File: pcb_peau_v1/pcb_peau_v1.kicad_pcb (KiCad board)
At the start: 2 copper layers, 76 x 75.7 mm, 27 parts, among them J1 Conn_01x05, J2 Conn_01x05, J3 Conn_01x02, J4 Conn_02x08_Top_Bottom, J5 Conn_02x12_Top_Bottom, U2 TLC274, U3 CD74HC4067SM, U4 CD74HC4067SM, U5 CD74HC4067SM, U6 CD74HC4067SM, U7 TLC274, U8 TLC274, U9 TLC274

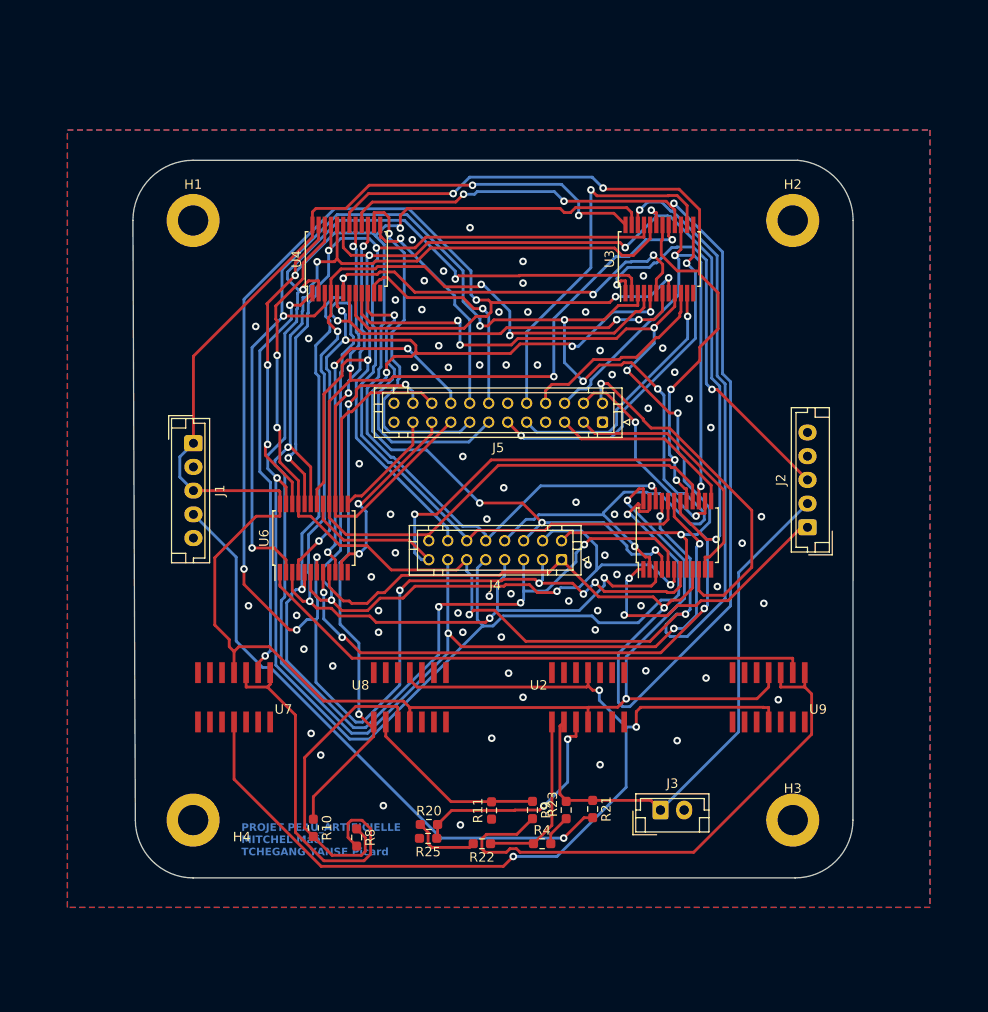
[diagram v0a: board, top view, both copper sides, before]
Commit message: pdb bulletproof
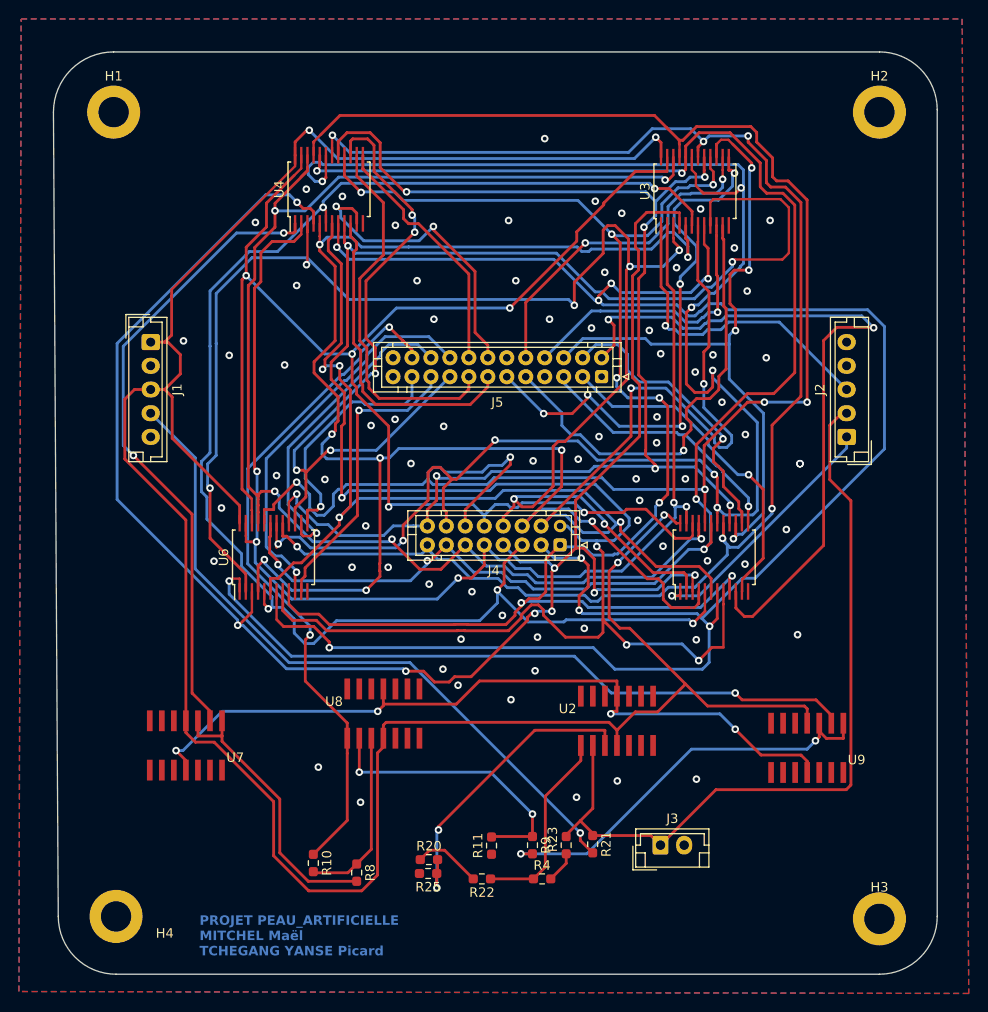
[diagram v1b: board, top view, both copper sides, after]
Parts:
- moved H2 14.6 mm to (247.7, 39.1)
- moved H1 14.2 mm to (166.9, 39.1)
- moved H3 13.9 mm to (247.7, 124.2)
- moved H4 13.0 mm to (167.1, 124.0)
- moved J1 11.6 mm to (170.8, 63.4)
- moved J2 10.4 mm to (244.2, 73.4)
- moved U3 8.07 mm to (228.2, 47.5)
- moved U4 7.58 mm to (189.6, 47.3)
- moved U7 7.18 mm to (174.5, 105.9)
- moved U9 6.71 mm to (240.0, 106.2)
- moved J5 4.79 mm to (218.3, 67.0)
- moved U6 4.71 mm to (183.7, 86.1)
- moved U5 4.54 mm to (230.2, 86.1)
- moved U2 3.93 mm to (220.0, 103.3)
- moved J3 3.71 mm to (224.6, 116.4)
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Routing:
- net Net-(J4-Pin_2): track 144.7 -> 210.5 mm, vias 9 -> 6
- net +5V: track 200.4 -> 262.6 mm
- net Net-(J4-Pin_7): track 128.8 -> 185.0 mm, vias 6 -> 8
- net Net-(J4-Pin_12): track 129.1 -> 180.2 mm, vias 3 -> 5
- net Net-(J4-Pin_14): track 138.5 -> 183.3 mm, vias 5 -> 9
- net Net-(J4-Pin_6): track 121.6 -> 166.0 mm, vias 9 -> 8
- net Net-(J4-Pin_9): track 170.2 -> 130.1 mm, vias 4 -> 5
- net A1: track 38.9 -> 76.4 mm, vias 1 -> 2
- net Net-(J4-Pin_4): track 133.0 -> 160.6 mm
- net AOP0IN+: track 57.9 -> 84.3 mm
- net Net-(J4-Pin_15): track 134.2 -> 159.7 mm
- net -5V: track 107.1 -> 81.7 mm, vias 3 -> 4
- net NE2: track 48.7 -> 73.1 mm, vias 2 -> 5
- net AOP1: track 44.1 -> 67.3 mm
- net B3: track 27.2 -> 47.9 mm
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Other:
- board size 76 x 75.7 mm -> 93.2 x 97.3 mm
